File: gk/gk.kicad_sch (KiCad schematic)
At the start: 58 parts, among them J1 USB_C_Receptacle_USB2.0, J10 Barrel_Jack_Switch, J2 Conn_01x02, J8 Conn_ARM_JTAG_SWD_10, U1 WE-TVS-82400102, U2 MCP73831-2-OT, U3 AP62300WU

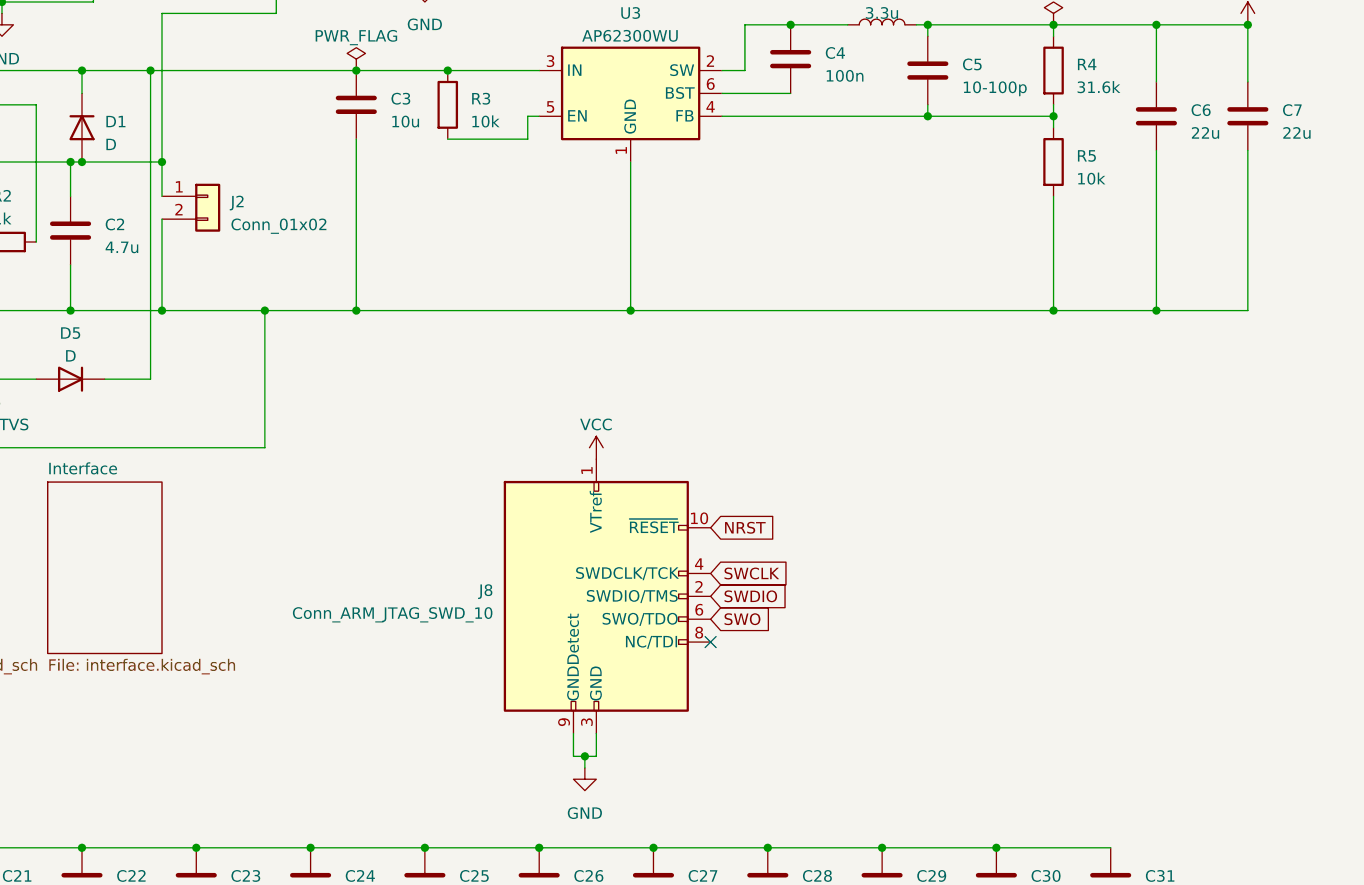
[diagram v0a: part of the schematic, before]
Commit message: Update pcb
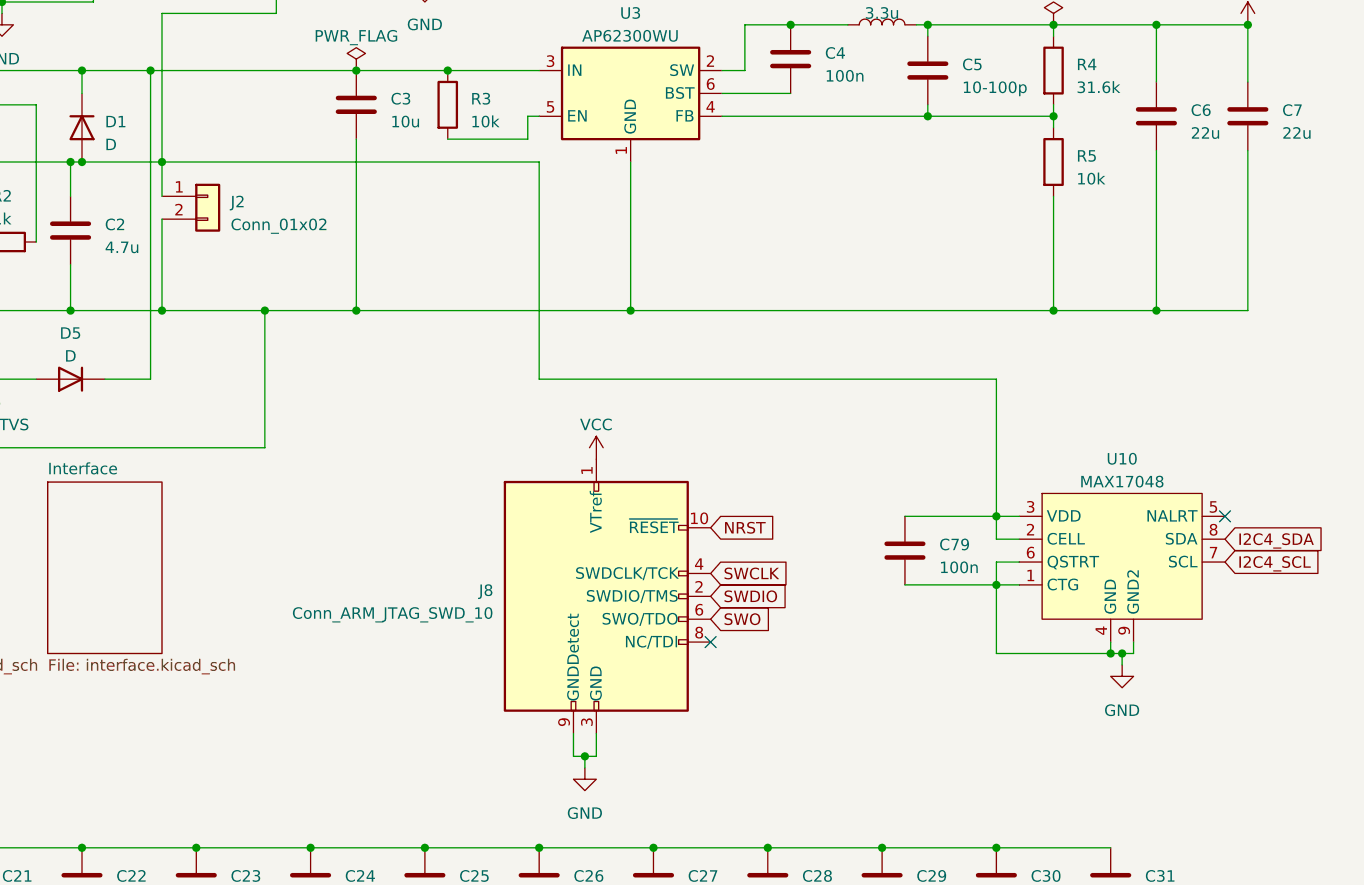
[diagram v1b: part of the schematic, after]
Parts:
- added C79: 100n, Capacitor_SMD:C_0603_1608Metric, symbol Device:C
- added U10: MAX17048, Package_DFN_QFN:TDFN-8-1EP_2x2mm_P0.5mm_EP0.8x1.2mm, symbol gk-syms:MAX17048
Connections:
- net GND: now also C79.2, U10.1 (CTG), U10.4 (GND), U10.6 (QSTRT), U10.9 (GND2)
- net at C2.1, D1.2 (A), J2.1 (Pin_1)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: now also C79.1, U10.2 (CELL), U10.3 (VDD)
- new net I2C4_SCL: U10.7 (SCL)
- new net I2C4_SDA: U10.8 (SDA)
- no-connect marks 3 -> 4
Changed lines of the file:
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@@
   (junction (at 63.5 53.34) (diameter 0) (color 0 0 0 0)
   )
+  (junction (at 240.03 95.25) (diameter 0) (color 0 0 0 0)
+  )
   (junction (at 124.46 80.01) (diameter 0) (color 0 0 0 0)
   )
@@
   (junction (at 113.03 139.7) (diameter 0) (color 0 0 0 0)
   )
+  (junction (at 252.73 110.49) (diameter 0) (color 0 0 0 0)
+  )
   (junction (at 217.17 40.64) (diameter 0) (color 0 0 0 0)
   )
@@
   (junction (at 62.23 132.08) (diameter 0) (color 0 0 0 0)
   )
+  (junction (at 254 110.49) (diameter 0) (color 0 0 0 0)
+  )
   (junction (at 138.43 132.08) (diameter 0) (color 0 0 0 0)
   )
@@
   (junction (at 201.93 132.08) (diameter 0) (color 0 0 0 0)
   )
+  (junction (at 240.03 102.87) (diameter 0) (color 0 0 0 0)
+  )
   (junction (at 227.33 139.7) (diameter 0) (color 0 0 0 0)
   )
@@
   )
   (no_connect (at 52.07 60.96))
+  (no_connect (at 265.43 95.25))
   (no_connect (at 52.07 63.5))
   (no_connect (at 208.28 109.22))
@@
     (stroke (width 0) (type default))
   )
+  (wire (pts (xy 240.03 95.25) (xy 242.57 95.25))
+    (stroke (width 0) (type default))
+  )
   (wire (pts (xy 36.83 71.12) (xy 36.83 72.39))
     (stroke (width 0) (type default))
@@
     (stroke (width 0) (type default))
   )
+  (wire (pts (xy 229.87 95.25) (xy 240.03 95.25))
+    (stroke (width 0) (type default))
+  )
+  (wire (pts (xy 242.57 102.87) (xy 240.03 102.87))
+    (stroke (width 0) (type default))
+  )
+  (wire (pts (xy 252.73 109.22) (xy 252.73 110.49))
+    (stroke (width 0) (type default))
+  )
   (wire (pts (xy 55.88 29.21) (xy 63.5 29.21))
     (stroke (width 0) (type default))
@@
     (stroke (width 0) (type default))
   )
+  (wire (pts (xy 255.27 110.49) (xy 254 110.49))
+    (stroke (width 0) (type default))
+  )
   (wire (pts (xy 137.16 72.39) (xy 147.32 72.39))
     (stroke (width 0) (type default))
@@
     (stroke (width 0) (type default))
   )
+  (wire (pts (xy 240.03 102.87) (xy 240.03 110.49))
+    (stroke (width 0) (type default))
+  )
+  (wire (pts (xy 242.57 100.33) (xy 240.03 100.33))
+    (stroke (width 0) (type default))
+  )
   (wire (pts (xy 166.37 25.4) (xy 166.37 26.67))
     (stroke (width 0) (type default))
@@
     (stroke (width 0) (type default))
   )
+  (wire (pts (xy 240.03 110.49) (xy 252.73 110.49))
+    (stroke (width 0) (type default))
+  )
   (wire (pts (xy 29.21 72.39) (xy 36.83 72.39))
     (stroke (width 0) (type default))
@@
     (stroke (width 0) (type default))
   )
+  (wire (pts (xy 147.32 55.88) (xy 189.23 55.88))
+    (stroke (width 0) (type default))
+  )
   (wire (pts (xy 113.03 139.7) (xy 125.73 139.7))
     (stroke (width 0) (type default))
@@
     (stroke (width 0) (type default))
   )
+  (wire (pts (xy 189.23 55.88) (xy 189.23 80.01))
+    (stroke (width 0) (type default))
+  )
   (wire (pts (xy 54.61 48.26) (xy 54.61 45.72))
     (stroke (width 0) (type default))
@@
     (stroke (width 0) (type default))
   )
+  (wire (pts (xy 240.03 80.01) (xy 240.03 95.25))
+    (stroke (width 0) (type default))
+  )
   (wire (pts (xy 76.2 29.21) (xy 76.2 21.59))
     (stroke (width 0) (type default))
@@
     (stroke (width 0) (type default))
   )
+  (wire (pts (xy 189.23 80.01) (xy 240.03 80.01))
+    (stroke (width 0) (type default))
+  )
   (wire (pts (xy 138.43 45.72) (xy 146.05 45.72))
     (stroke (width 0) (type default))
@@
     (stroke (width 0) (type default))
   )
+  (wire (pts (xy 229.87 102.87) (xy 240.03 102.87))
+    (stroke (width 0) (type default))
+  )
   (wire (pts (xy 78.74 53.34) (xy 82.55 53.34))
     (stroke (width 0) (type default))
@@
     (stroke (width 0) (type default))
   )
+  (wire (pts (xy 252.73 110.49) (xy 254 110.49))
+    (stroke (width 0) (type default))
+  )
   (wire (pts (xy 232.41 50.8) (xy 232.41 49.53))
     (stroke (width 0) (type default))
@@
     (stroke (width 0) (type default))
   )
+  (wire (pts (xy 240.03 97.79) (xy 240.03 95.25))
+    (stroke (width 0) (type default))
+  )
   (wire (pts (xy 217.17 40.64) (xy 223.52 40.64))
     (stroke (width 0) (type default))
@@
     (stroke (width 0) (type default))
   )
+  (wire (pts (xy 242.57 97.79) (xy 240.03 97.79))
+    (stroke (width 0) (type default))
+  )
   (wire (pts (xy 81.28 50.8) (xy 81.28 72.39))
     (stroke (width 0) (type default))
@@
     (stroke (width 0) (type default))
   )
+  (wire (pts (xy 254 110.49) (xy 254 111.76))
+    (stroke (width 0) (type default))
+  )
+  (wire (pts (xy 255.27 109.22) (xy 255.27 110.49))
+    (stroke (width 0) (type default))
+  )
   (wire (pts (xy 147.32 55.88) (xy 147.32 39.37))
     (stroke (width 0) (type default))
@@
   )
   (wire (pts (xy 55.88 40.64) (xy 55.88 29.21))
+    (stroke (width 0) (type default))
+  )
+  (wire (pts (xy 240.03 100.33) (xy 240.03 102.87))
     (stroke (width 0) (type default))
   )
@@
     )
   )
+  (global_label "I2C4_SCL" (shape input) (at 265.43 100.33 0) (fields_autoplaced)
+    (effects (font (size 1.27 1.27)) (justify left))
+    (property "Intersheetrefs" "${INTERSHEET_REFS}" (at 277.1048 100.33 0)
+      (effects (font (size 1.27 1.27)) (justify left) hide)
+    )
+  )
   (global_label "USB_VBUS" (shape input) (at 102.87 33.02 0) (fields_autoplaced)
     (effects (font (size 1.27 1.27)) (justify left))
@@
     )
   )
+  (global_label "I2C4_SDA" (shape input) (at 265.43 97.79 0) (fields_autoplaced)
+    (effects (font (size 1.27 1.27)) (justify left))
+    (property "Intersheetrefs" "${INTERSHEET_REFS}" (at 277.1653 97.79 0)
+      (effects (font (size 1.27 1.27)) (justify left) hide)
+    )
+  )
   (global_label "SWCLK" (shape input) (at 208.28 101.6 0) (fields_autoplaced)
     (effects (font (size 1.27 1.27)) (justify left))
@@
         (path "/08730ac6-6084-459f-bdf1-86b322355ede"
           (reference "#FLG03") (unit 1)
+        )
+      )
+    )
+  )
+  (symbol (lib_id "power:GND") (at 254 111.76 0) (unit 1)
+    (in_bom yes) (on_board yes) (dnp no) (fields_autoplaced)
+    (property "Reference" "#PWR071" (at 254 118.11 0)
+      (effects (font (size 1.27 1.27)) hide)
+    )
+    (property "Value" "GND" (at 254 116.84 0)
+      (effects (font (size 1.27 1.27)))
+    )
+    (property "Footprint" "" (at 254 111.76 0)
+      (effects (font (size 1.27 1.27)) hide)
+    )
+    (property "Datasheet" "" (at 254 111.76 0)
+      (effects (font (size 1.27 1.27)) hide)
+    )
+    (pin "1")
+    (instances
+      (project "gk"
+        (path "/08730ac6-6084-459f-bdf1-86b322355ede"
+          (reference "#PWR071") (unit 1)
         )
       )
@@
     )
   )
+  (symbol (lib_id "Device:C") (at 229.87 99.06 0) (unit 1)
+    (in_bom yes) (on_board yes) (dnp no) (fields_autoplaced)
+    (property "Reference" "C79" (at 233.68 98.425 0)
+      (effects (font (size 1.27 1.27)) (justify left))
+    )
+    (property "Value" "100n" (at 233.68 100.965 0)
+      (effects (font (size 1.27 1.27)) (justify left))
+    )
+    (property "Footprint" "Capacitor_SMD:C_0603_1608Metric" (at 230.8352 102.87 0)
+      (effects (font (size 1.27 1.27)) hide)
+    )
+    (property "Datasheet" "~" (at 229.87 99.06 0)
+      (effects (font (size 1.27 1.27)) hide)
+    )
+    (pin "1")
+    (pin "2")
+    (instances
+      (project "gk"
+        (path "/08730ac6-6084-459f-bdf1-86b322355ede"
+          (reference "C79") (unit 1)
+        )
+      )
+    )
+  )
   (symbol (lib_id "power:GND") (at 176.53 35.56 0) (unit 1)
     (in_bom yes) (on_board yes) (dnp no) (fields_autoplaced)
@@
         )
       )
+    )
+  )
+  (symbol (lib_id "gk-syms:MAX17048") (at 254 90.17 0) (unit 1)
+    (in_bom yes) (on_board yes) (dnp no) (fields_autoplaced)
+    (property "Reference" "U10" (at 254 88.9 0)
+      (effects (font (size 1.27 1.27)))
+    )
+    (property "Value" "MAX17048" (at 254 91.44 0)
+      (effects (font (size 1.27 1.27)))
+    )
+    (property "Footprint" "Package_DFN_QFN:TDFN-8-1EP_2x2mm_P0.5mm_EP0.8x1.2mm" (at 254 91.44 0)
+      (effects (font (size 1.27 1.27)) hide)
+    )
+    (property "Datasheet" "" (at 254 90.17 0)
+      (effects (font (size 1.27 1.27)) hide)
+    )
+    (pin "1")
+    (pin "2")
+    (pin "3")
+    (pin "4")
+    (pin "5")
+    (pin "6")
+    (pin "7")
+    (pin "8")
+    (pin "9")
+    (instances
+      (project "gk"
+        (path "/08730ac6-6084-459f-bdf1-86b322355ede"
+          (reference "U10") (unit 1)
+        )
+      )
